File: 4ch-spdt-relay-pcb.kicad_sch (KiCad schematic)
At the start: 33 parts, among them J1 Screw_Terminal_01x03, J2 Conn_01x06_Pin, J3 Screw_Terminal_01x03, J4 Screw_Terminal_01x03, J5 Screw_Terminal_01x03, K1 G5LE-1, K2 G5LE-1, K3 G5LE-1, K4 G5LE-1, Q1 2N3904, Q2 2N3904, Q3 2N3904, Q4 2N3904

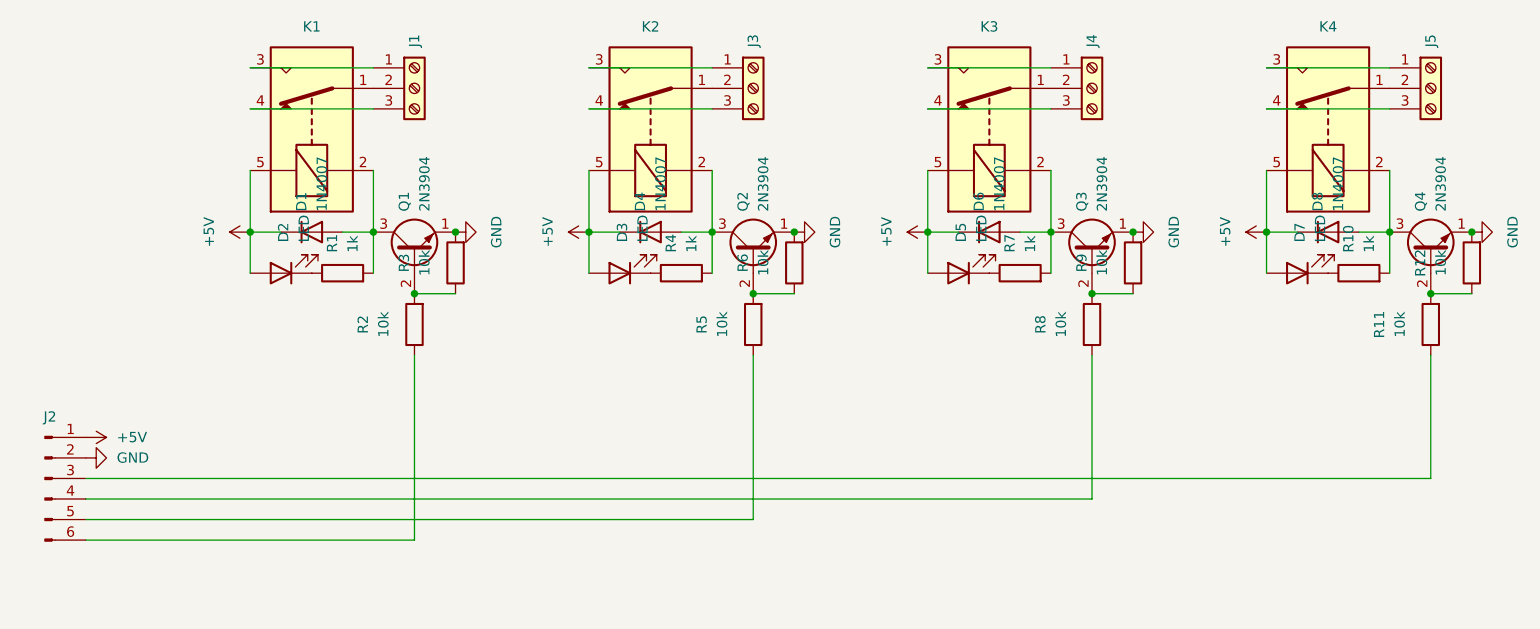
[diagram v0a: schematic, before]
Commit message: Add files via upload
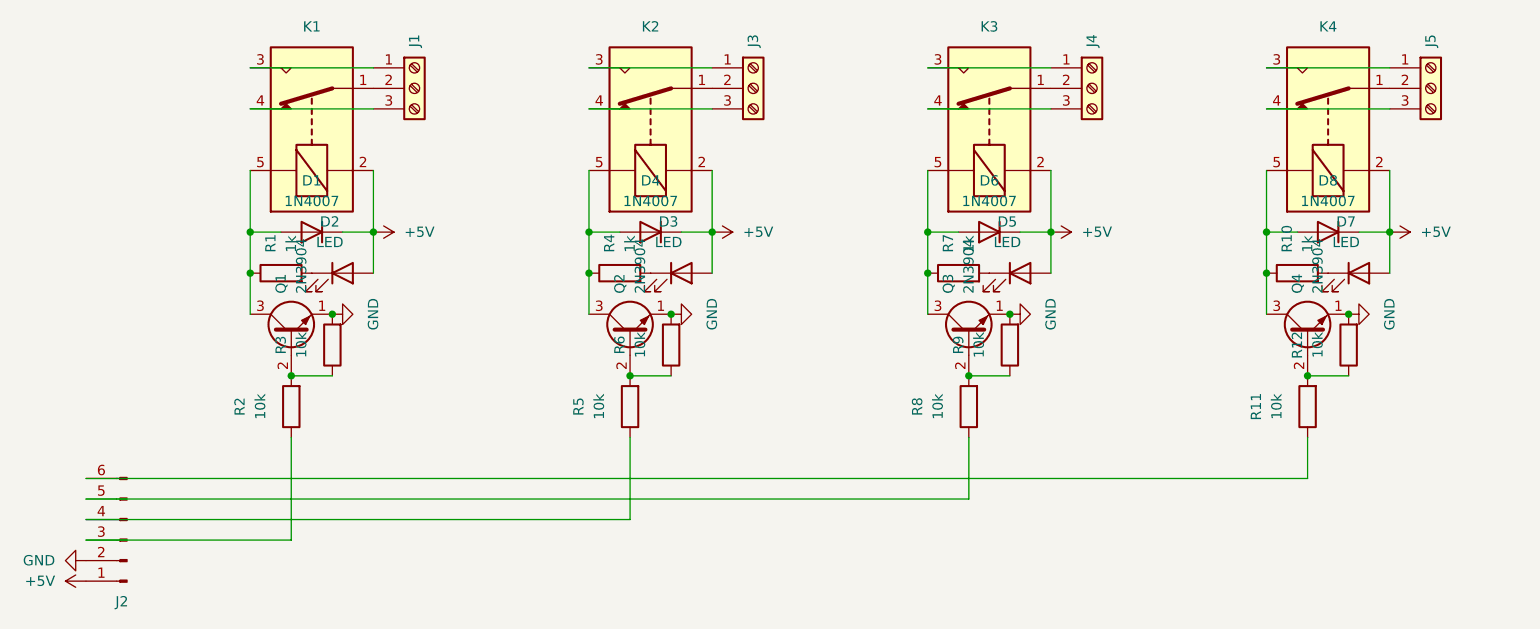
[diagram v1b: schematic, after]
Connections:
- net +5V: now also K1.2, K2.2, K3.2, K4.2; no longer K1.5, K2.5, K3.5, K4.5
- net at D6.2 (A), Q3.3 (C): now also K3.5, R7.1; no longer K3.2, R7.2
- net at D8.2 (A), Q4.3 (C): now also K4.5, R10.1; no longer K4.2, R10.2
- net at R4.1: now also D4.2 (A), K2.5, Q2.3 (C); no longer D3.1 (K)
- net at D1.2 (A), Q1.3 (C): now also K1.5, R1.1; no longer K1.2, R1.2
- net at D2.1 (K): now also R1.2; no longer R1.1
- net at D7.1 (K): now also R10.2; no longer R10.1
- net at R11.1: now also J2.6 (Pin_6); no longer J2.3 (Pin_3)
- net at R2.1: now also J2.3 (Pin_3); no longer J2.6 (Pin_6)
- net at J2.4 (Pin_4): now also R5.1; no longer R8.1
- net at J2.5 (Pin_5): now also R8.1; no longer R5.1
- net at D5.1 (K): now also R7.2; no longer R7.1
- new net: D3.1 (K), R4.2
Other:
- moved on the sheet: D1, D2, D4, D5, D7, D8, J2, Q1, Q2, Q3, Q4, R1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
